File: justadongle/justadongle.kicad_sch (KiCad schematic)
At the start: 26 parts, among them U1 SL2.1A_C6798314, U2 FSUSB42MUX, U3 LMV7219M5X/NOPB, U4 HC-USB3.0-C26

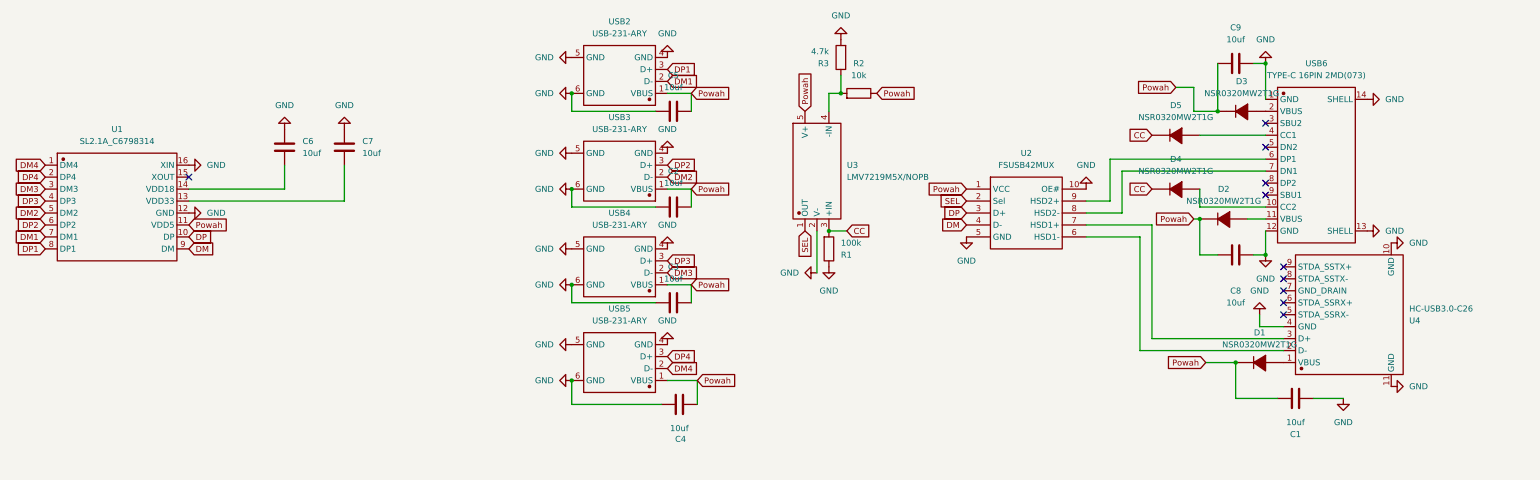
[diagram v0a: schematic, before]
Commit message: Finished the Board
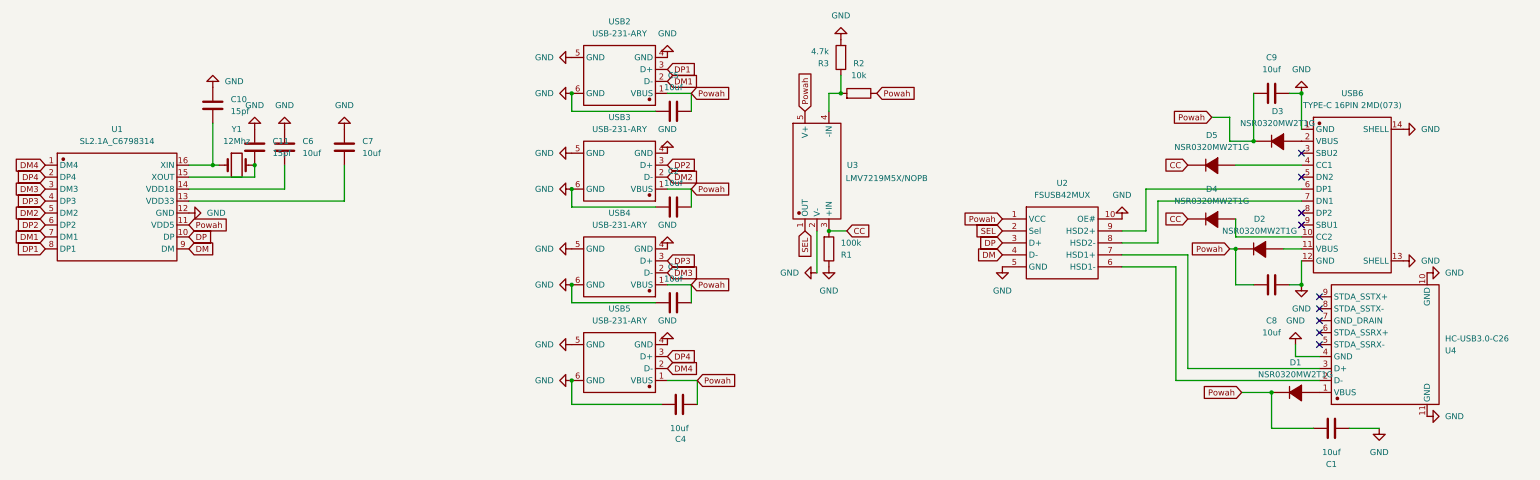
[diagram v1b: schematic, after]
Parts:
- added C10, C11: 15pf, Footprints:CAP-TH_BD5.0-P2.00-D0.8-FD, symbol Device:C
- added Y1: 12Mhz, easyeda2kicad:CRYSTAL-SMD_4P-L3.2-W2.5-BL, symbol Device:Crystal
- C1, C2, C3, C4, C5, C6, C7, C8, C9: footprint Footprints:CAP-TH_BD5.0-P2.00-D0.8-FD -> easyeda2kicad:C0805
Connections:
- net GND: now also C10.1, C11.1; no longer U1.16 (XIN)
- net at U1.15 (XOUT): now also C11.2, Y1.2
- new net: C10.2, U1.16 (XIN), Y1.1
- no-connect marks 10 -> 9
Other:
- moved on the sheet: C1, C8, C9, D1, D2, D3, D4, D5, U2, U4, USB6
